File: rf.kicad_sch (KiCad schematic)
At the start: 7 parts, among them U3 MAX-M10S, Y1 ECS-TXO-25CSMV-320-AM-TR

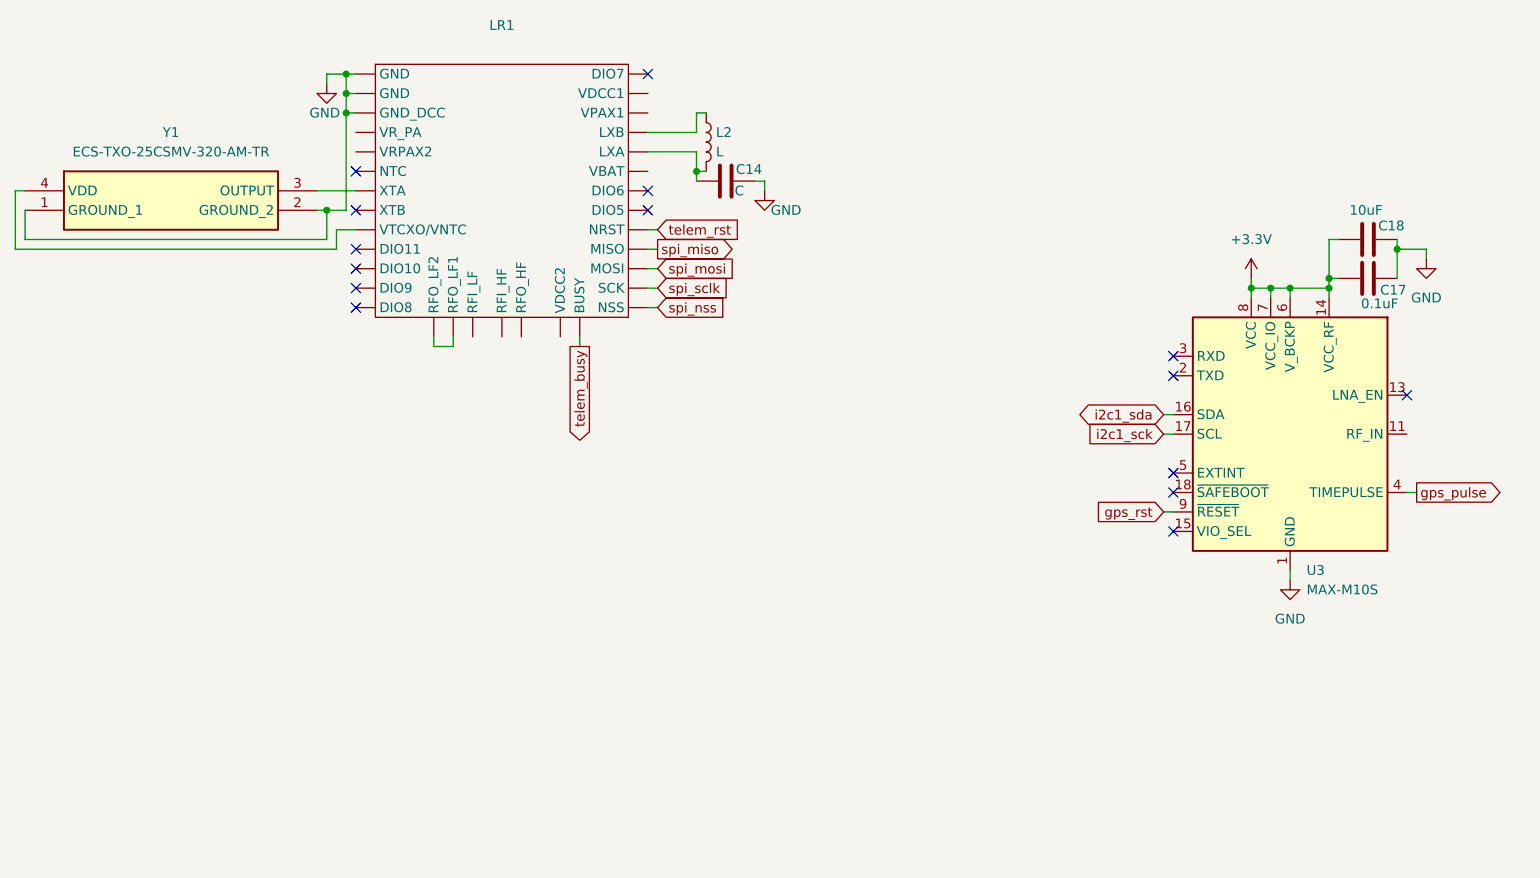
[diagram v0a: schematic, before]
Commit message: oops forgot to commit - looks like I worked on the lr2021's symbol and the schematic - see journal for details on what I did
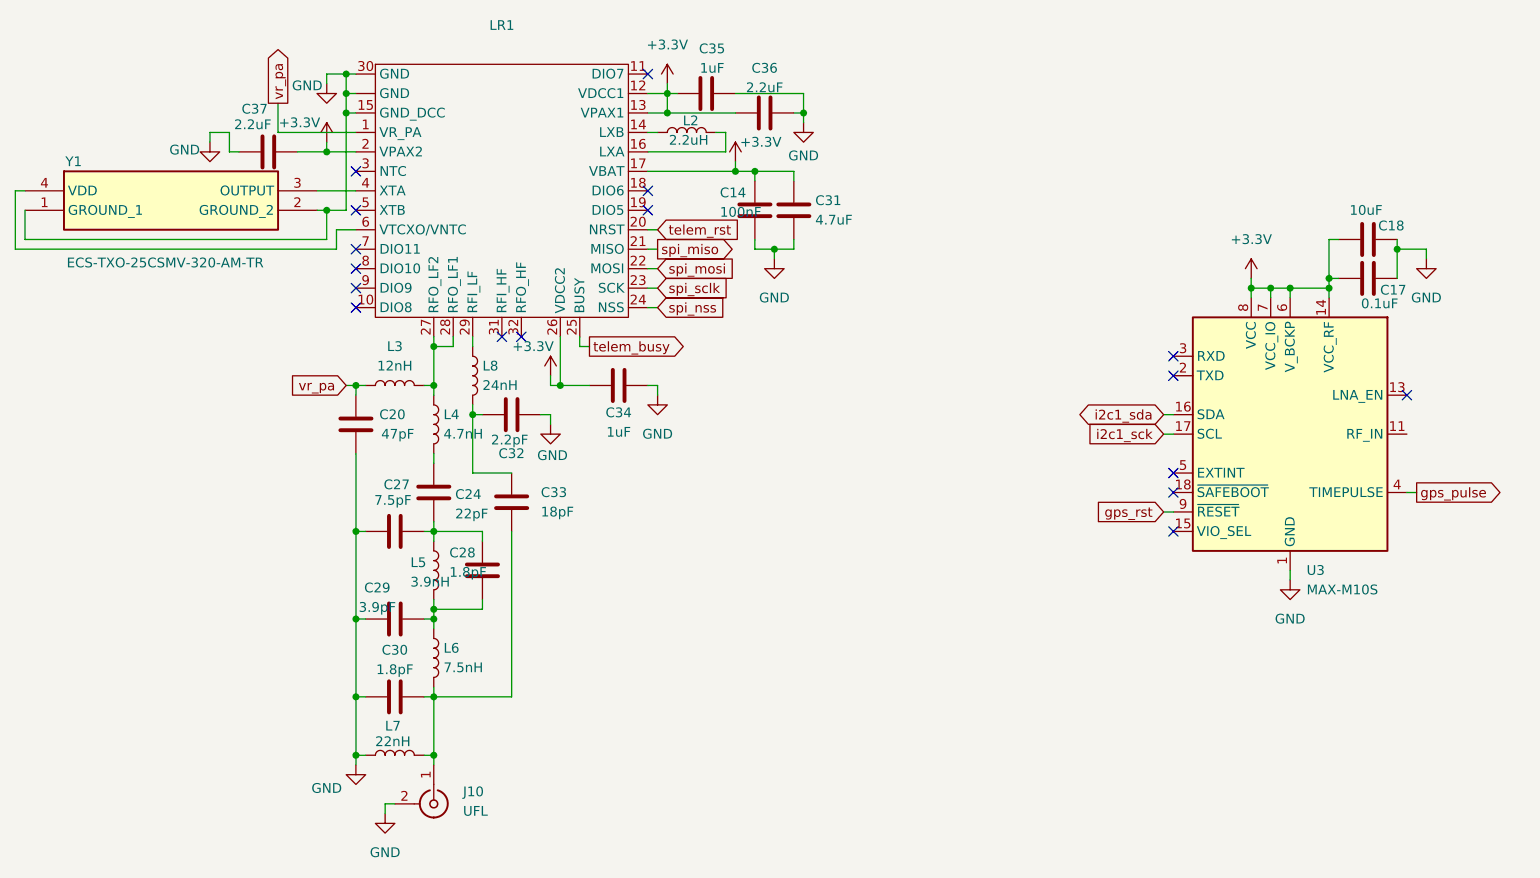
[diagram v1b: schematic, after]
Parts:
- added C20: 47pF, symbol Device:C
- added C24: 22pF, symbol Device:C
- added C27: 7.5pF, symbol Device:C
- added C28, C30: 1.8pF, symbol Device:C
- added C29: 3.9pF, symbol Device:C
- added C31: 4.7uF, symbol Device:C
- added C32: 2.2pF, symbol Device:C
- added C33: 18pF, symbol Device:C
- added C34, C35: 1uF, symbol Device:C
- added C36, C37: 2.2uF, symbol Device:C
- added J10: UFL, symbol Connector:Conn_Coaxial
- added L3: 12nH, symbol Device:L
- added L4: 4.7nH, symbol Device:L
- added L5: 3.9nH, symbol Device:L
- added L6: 7.5nH, symbol Device:L
- added L7: 22nH, symbol Device:L
- added L8: 24nH, symbol Device:L
- C14: value C -> 100nF
- L2: value L -> 2.2uH
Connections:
- net +3.3V: now also C14.1, LR1.12 (VDCC1), LR1.13 (VPAX1), LR1.17 (VBAT), LR1.2 (VPAX2), LR1.26 (VDCC2), C31.1, C34.1, C35.1, C36.1, C37.2
- net GND: now also LR1.15 (GND_DCC), LR1.30 (GND), C20.2, C27.1, C29.1, C30.1, C31.2, C32.2, C34.2, C35.2, C36.2, C37.1, J10.2 (Ext), L7.1
- net spi_miso: now also LR1.21 (MISO); no longer LR1. (NSS)
- net spi_mosi: now also LR1.22 (MOSI); no longer LR1. (NSS)
- net spi_nss: now also LR1.24 (NSS); no longer LR1. (NSS)
- net spi_sclk: now also LR1.23 (SCK); no longer LR1. (NSS)
- net telem_busy: now also LR1.25 (BUSY); no longer LR1. (NSS)
- net telem_rst: now also LR1.20 (NRST); no longer LR1. (NSS)
- net at Y1.3 (OUTPUT): now also LR1.4 (XTA); no longer LR1. (NSS)
- net at Y1.4 (VDD): now also LR1.6 (VTCXO/VNTC); no longer LR1. (NSS)
- net at L2.1: now also LR1.14 (LXB); no longer LR1. (NSS)
- new net: C30.2, C33.2, J10.1 (In), L6.2, L7.2
- new net: C24.1, L4.2
- new net: C24.2, C27.2, C28.1, L5.1
- new net: L3.2, L4.1, LR1.27 (RFO_LF2), LR1.28 (RFO_LF1)
- new net: C28.2, C29.2, L5.2, L6.1
- new net: C32.1, C33.1, L8.2
- new net: L8.1, LR1.29 (RFI_LF)
- new net: L2.2, LR1.16 (LXA)
- new net vr_pa: C20.1, L3.1, LR1.1 (VR_PA)
- no-connect marks 15 -> 17
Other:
- moved on the sheet: L2

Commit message: tons of progress on schematic and pcb - see journal for details
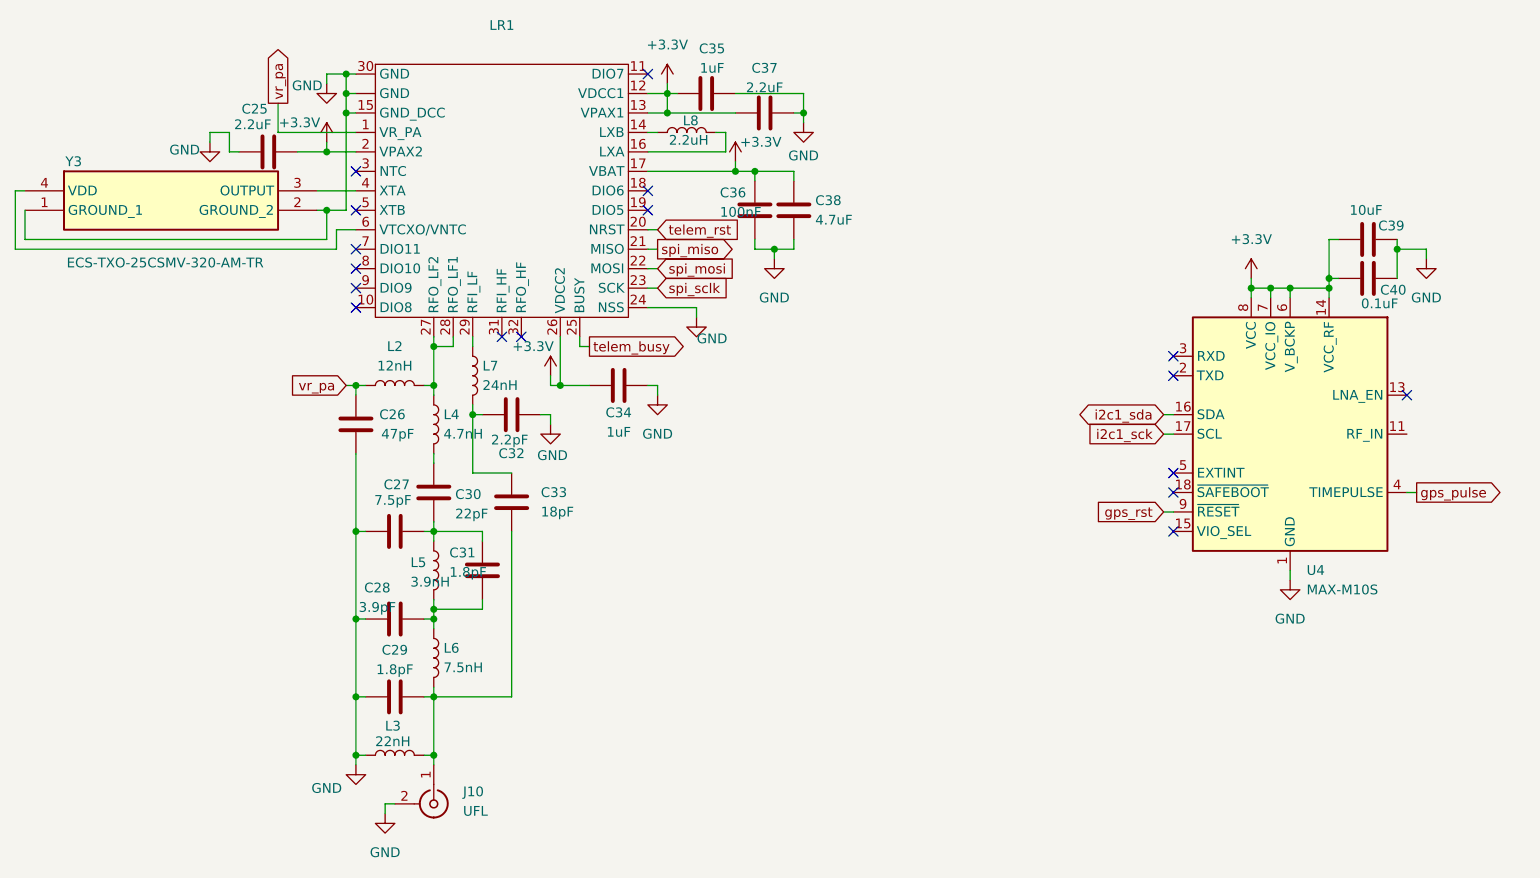
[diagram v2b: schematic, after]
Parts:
- C25: renamed from C37; footprint (none) -> Capacitor_SMD:C_0603_1608Metric
- C26: renamed from C20; footprint (none) -> Capacitor_SMD:C_0402_1005Metric
- C27, C32, C33: footprint (none) -> Capacitor_SMD:C_0402_1005Metric
- C28: renamed from C29; footprint (none) -> Capacitor_SMD:C_0402_1005Metric
- C29: renamed from C30; footprint (none) -> Capacitor_SMD:C_0402_1005Metric
- C30: renamed from C24; footprint (none) -> Capacitor_SMD:C_0402_1005Metric
- C31: renamed from C28; footprint (none) -> Capacitor_SMD:C_0402_1005Metric
- C34, C35: footprint (none) -> Capacitor_SMD:C_0603_1608Metric
- C36: renamed from C14; footprint (none) -> Capacitor_SMD:C_0402_1005Metric
- C37: renamed from C36; footprint (none) -> Capacitor_SMD:C_0603_1608Metric
- C38: renamed from C31; footprint (none) -> Capacitor_SMD:C_0603_1608Metric
- L2: renamed from L3; footprint (none) -> Inductor_SMD:L_0402_1005Metric
- L3: renamed from L7; footprint (none) -> Inductor_SMD:L_0402_1005Metric
- L4, L5, L6: footprint (none) -> Inductor_SMD:L_0402_1005Metric
- L7: renamed from L8; footprint (none) -> Inductor_SMD:L_0402_1005Metric
- L8: renamed from L2; footprint (none) -> Inductor_SMD:L_0402_1005Metric
- LR1: footprint (none) -> footprints:Untitled
- Y3: renamed from Y1; footprint ECSTXO25CSMV320AMTR -> footprints:ECSTXO25CSMV320AMTR
- renumbered C18 to C39, C17 to C40, U3 to U4
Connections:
- net spi_nss is gone; now on net GND: LR1.24 (NSS)
